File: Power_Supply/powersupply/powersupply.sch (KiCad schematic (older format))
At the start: 45 parts

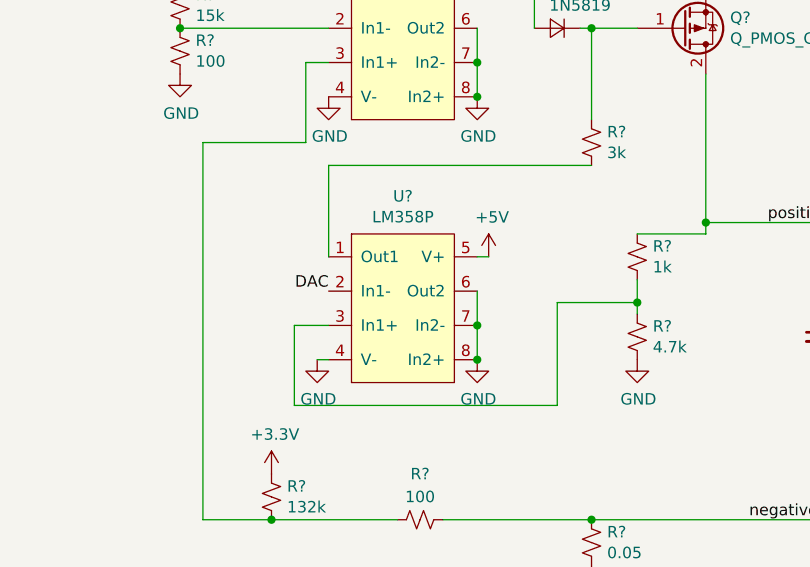
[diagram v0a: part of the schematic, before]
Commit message: small change
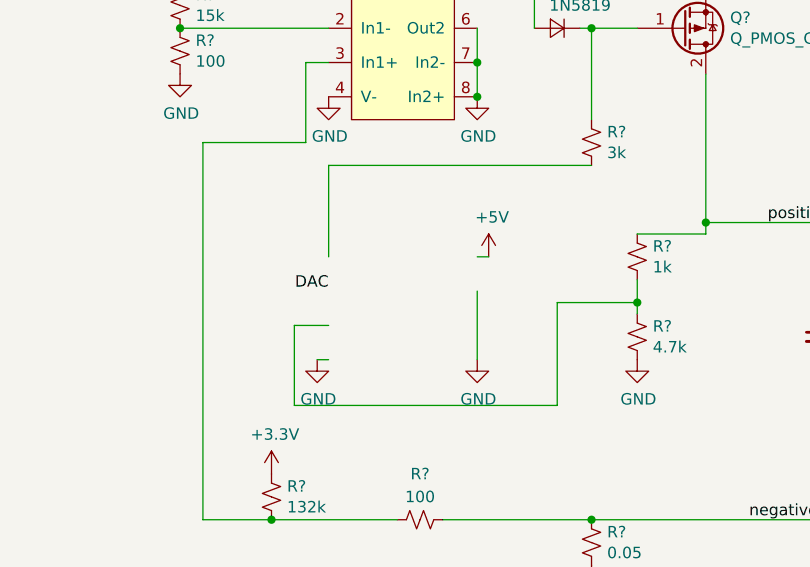
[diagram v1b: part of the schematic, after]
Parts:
- removed U?: LM358P, symbol powersupply:LM358P
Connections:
- wire segments 93 -> 92
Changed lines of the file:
@@
-$EndComp
-$Comp
-L powersupply:LM358P U?
-U 1 1 5D4AA099
-P 8400 4300
-F 0 "U?" H 8375 4415 50  0000 C CNN
-F 1 "LM358P" H 8375 4324 50  0000 C CNN
-F 2 "" H 8400 4300 50  0001 C CNN
-F 3 "" H 8400 4300 50  0001 C CNN
-	1    8400 4300
-	1    0    0    -1
 $EndComp
 $Comp
@@
 	1    0    0    -1
 $EndComp
-$Comp
-L Device:R_Small_US R?
-U 1 1 5D4C174A
-P 8450 5600
-F 0 "R?" V 8650 5600 50  0000 C CNN
-F 1 "100" V 8550 5600 50  0000 C CNN
-F 2 "" H 8450 5600 50  0001 C CNN
-F 3 "~" H 8450 5600 50  0001 C CNN
-	1    8450 5600
-	0    -1   -1   0
-$EndComp
 Wire Wire Line
 	8050 3600 7950 3600
@@
 Wire Wire Line
 	9050 4650 9050 5100
-Wire Wire Line
-	9050 5100 7900 5100
 Wire Wire Line
 	7900 5100 7900 4750
@@
 Connection ~ 8700 3750
 Connection ~ 8700 3600
-Wire Wire Line
-	8700 4600 8700 4750
-Wire Wire Line
-	8700 4900 8700 4750
-Connection ~ 8700 4750
 $Comp
 L power:GND #PWR?
@@
 	1    0    0    -1
 $EndComp
-Connection ~ 8700 4900
 $Comp
 L Device:L_Small L?
@@
 Wire Wire Line
 	7500 5600 7800 5600
-Connection ~ 7800 5600
-Wire Wire Line
-	7800 5600 8350 5600
-Wire Wire Line
-	8550 5600 9200 5600
-Connection ~ 9200 5600
 Wire Wire Line
 	10200 4900 10200 5600
@@
 Wire Wire Line
 	6600 2050 6800 2050
+Connection ~ 9200 5600
+Wire Wire Line
+	8550 5600 9200 5600
+Connection ~ 7800 5600
+Wire Wire Line
+	7800 5600 8350 5600
+Wire Wire Line
+	9050 5100 7900 5100
+$Comp
+L Device:R_Small_US R?
+U 1 1 5D4C174A
+P 8450 5600
+F 0 "R?" V 8650 5600 50  0000 C CNN
+F 1 "100" V 8550 5600 50  0000 C CNN
+F 2 "" H 8450 5600 50  0001 C CNN
+F 3 "~" H 8450 5600 50  0001 C CNN
+	1    8450 5600
+	0    -1   -1   0
+$EndComp
+Wire Wire Line
+	8700 4600 8700 4900
 $EndSCHEMATC
